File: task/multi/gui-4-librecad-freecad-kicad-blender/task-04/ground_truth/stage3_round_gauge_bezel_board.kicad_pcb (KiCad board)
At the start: 118 x 118 mm, 0 parts

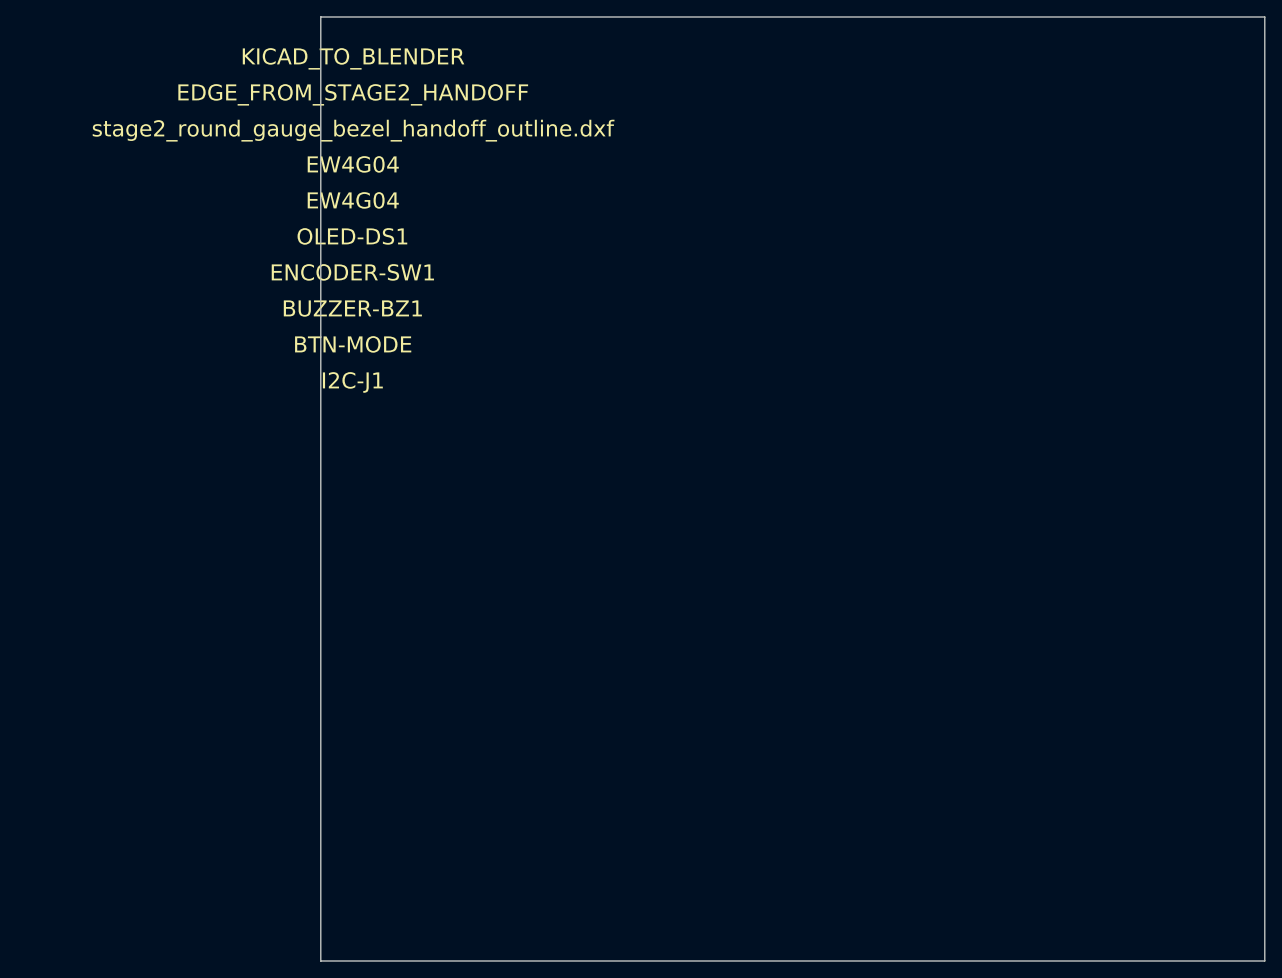
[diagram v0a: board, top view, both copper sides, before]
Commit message: 更新修复后的正式 task 数据
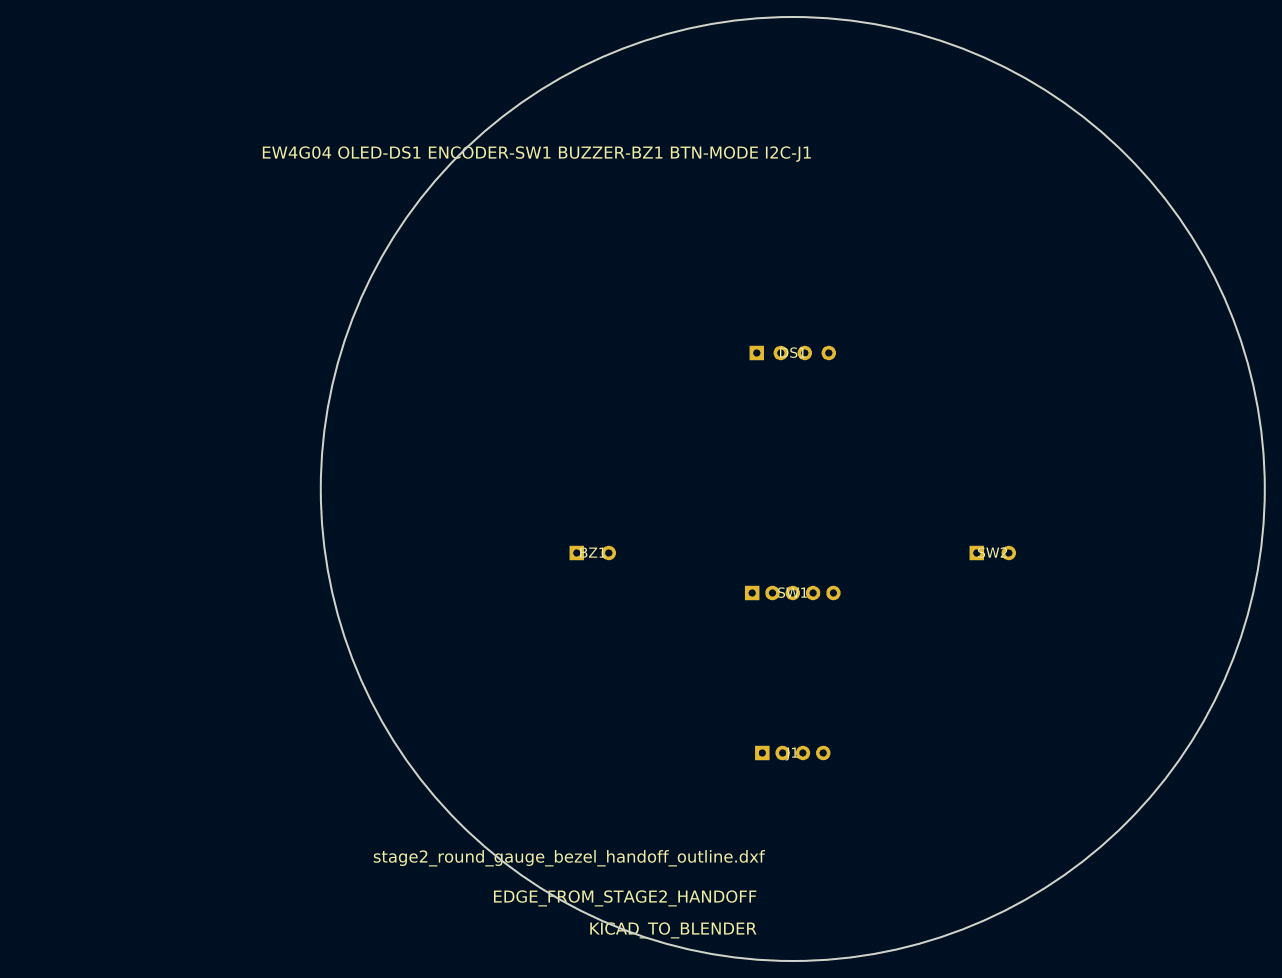
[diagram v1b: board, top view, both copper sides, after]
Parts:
- added BZ1: Gauge Buzzer, , F.Cu at (34.0, 67.0)
- added DS1: OLED Display, , F.Cu at (59.0, 42.0)
- added J1: I2C Header, , F.Cu at (59.0, 92.0)
- added SW1: Rotary Encoder, , F.Cu at (59.0, 72.0)
- added SW2: Mode Button, , F.Cu at (84.0, 67.0)
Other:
- outline, holes or cut-outs redrawn
- copper layers 0 -> 2
- board text added: "EW4G04 OLED-DS1 ENCODER-SW1 BUZZER-BZ1 BTN-MODE I2C-J1"
- board text removed: "BTN-MODE"
- board text removed: "BUZZER-BZ1"
- board text removed: "ENCODER-SW1"
- board text removed: "EW4G04"
- board text removed: "I2C-J1"
- board text removed: "OLED-DS1"
